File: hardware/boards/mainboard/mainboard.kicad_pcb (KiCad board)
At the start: 2 copper layers, 64.9 x 65 mm, 4 parts, among them J1 Conn_01x03, U1 RP2040

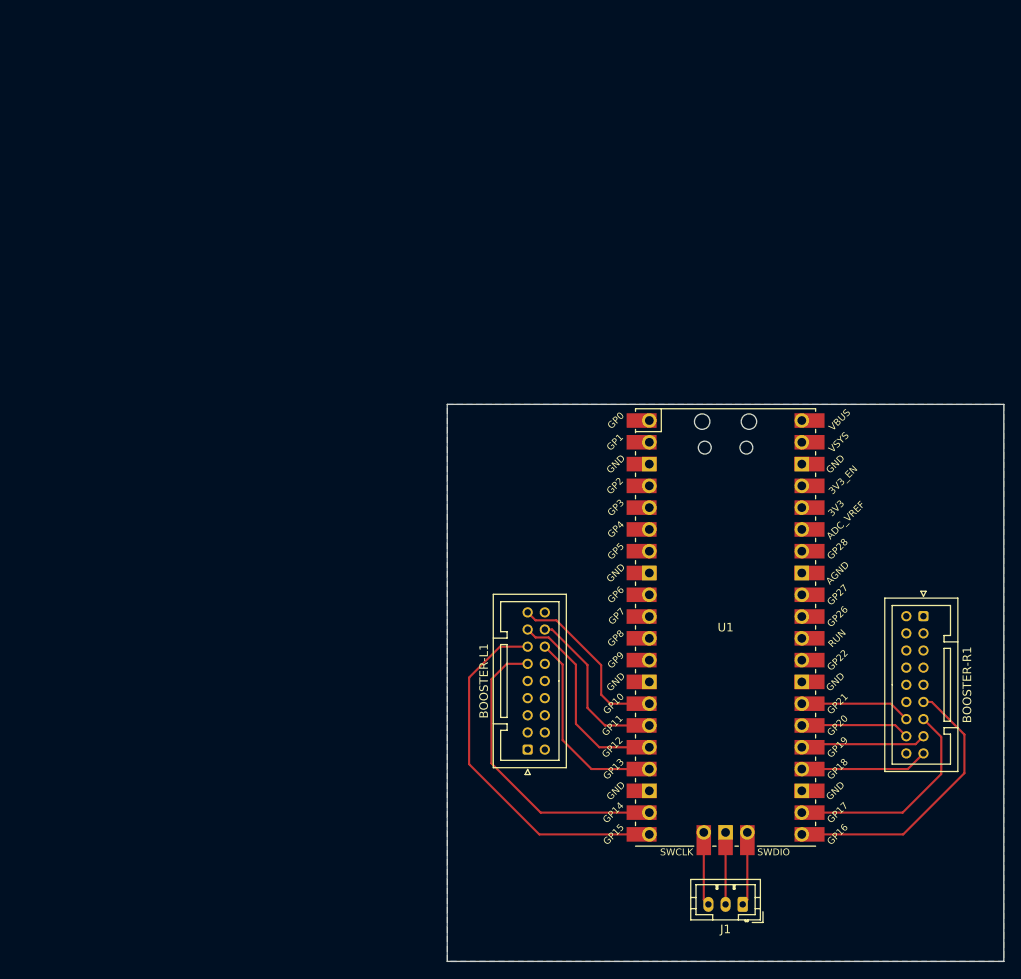
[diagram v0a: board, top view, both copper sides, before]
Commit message: refactor(hardware): refactor mainboard
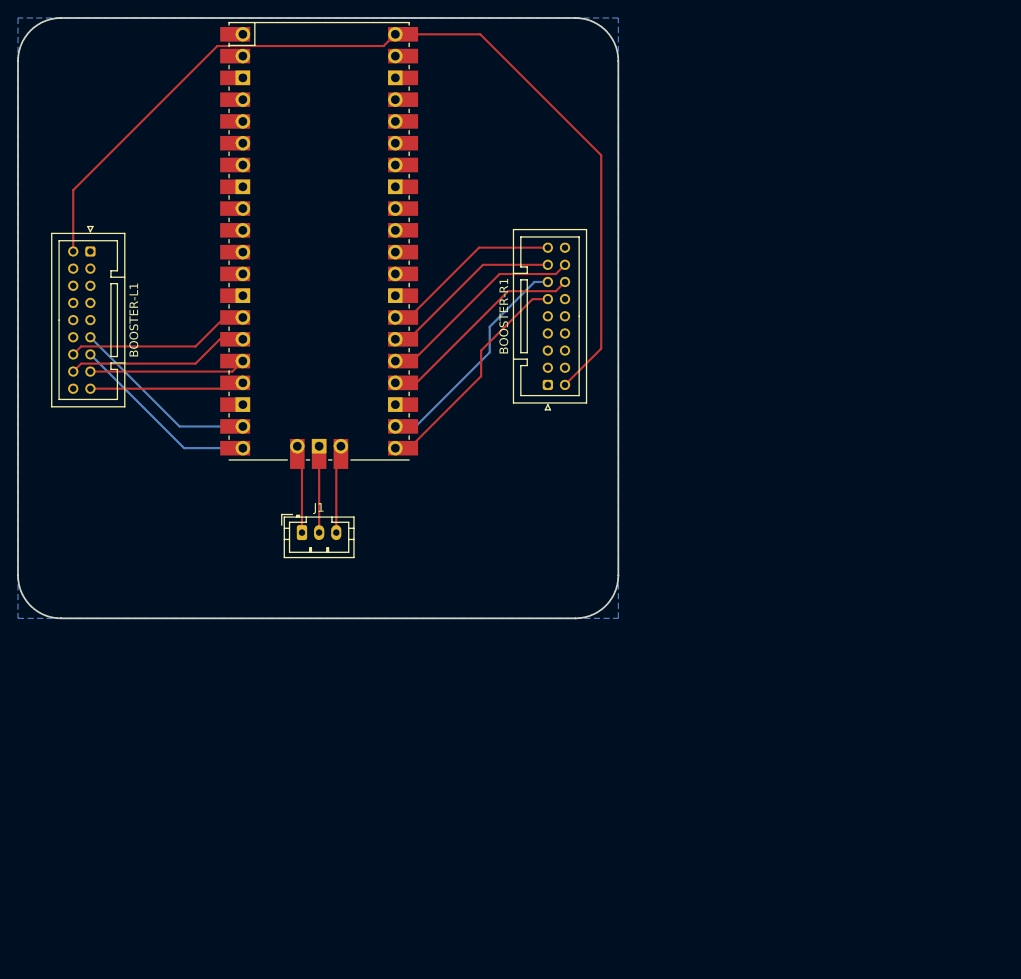
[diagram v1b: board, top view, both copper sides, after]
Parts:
- removed U1: RP2040, MCU_RaspberryPi_and_Boards:RPi_Pico_SMD_TH
- added U2: Pico, MCU_RaspberryPi_and_Boards:RPi_Pico_SMD_TH_Clean, F.Cu at (75.1, 66.0)
- moved BOOSTER-L1 77.3 mm to (48.4, 67.2), turned to -90 degrees
- moved J1 67.2 mm to (73.1, 100.0), turned to 0 degrees
- moved BOOSTER-R1 51.4 mm to (101.8, 82.8), turned to 90 degrees
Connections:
- net BOOSTER_L_SCL+ renamed /BOOSTER_L_SCL+
- net BOOSTER_L_SCL- renamed /BOOSTER_L_SCL-
- net BOOSTER_L_SDA+ renamed /BOOSTER_L_SDA+
- net BOOSTER_L_SDA- renamed /BOOSTER_L_SDA-
- BOOSTER-L1 pad 11: BOOSTER_L_BTN -> /BOOSTER_L_BTN
- BOOSTER-L1 pad 13: BOOSTER_L_BTN_LED -> /BOOSTER_L_BTN_LED
- BOOSTER-L1 pad 14: BOOSTER_L_DIR_4 -> /BOOSTER_L_DIR_4
- BOOSTER-L1 pad 15: BOOSTER_L_DIR_2 -> /BOOSTER_L_DIR_2
- BOOSTER-L1 pad 16: BOOSTER_L_DIR_3 -> /BOOSTER_L_DIR_3
- BOOSTER-L1 pad 17: BOOSTER_L_DIR_1 -> /BOOSTER_L_DIR_1
- BOOSTER-R1 pad 11: BOOSTER_R_BTN -> /BOOSTER_R_BTN
- BOOSTER-R1 pad 13: BOOSTER_R_BTN_LED -> /BOOSTER_R_BTN_LED
- BOOSTER-R1 pad 14: BOOSTER_R_DIR_4 -> /BOOSTER_R_DIR_4
- BOOSTER-R1 pad 15: BOOSTER_R_DIR_2 -> /BOOSTER_R_DIR_2
- BOOSTER-R1 pad 16: BOOSTER_R_DIR_3 -> /BOOSTER_R_DIR_3
- BOOSTER-R1 pad 17: BOOSTER_R_DIR_1 -> /BOOSTER_R_DIR_1
- J1 pad 1: DBG_SWCLK -> /DBG_SWCLK
- J1 pad 2: DBG_GND -> /DBG_GND
- J1 pad 3: DBG_SWDIO -> /DBG_SWDIO
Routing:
- net +5V: track 0.00 -> 110.6 mm
- net BOOSTER_L_BTN_LED: track 42.8 -> 0.00 mm
- net BOOSTER_L_BTN: track 35.6 -> 0.00 mm
- net BOOSTER_R_BTN: track 32.8 -> 0.00 mm
- net /BOOSTER_R_BTN: track 0.00 -> 26.7 mm
- net /BOOSTER_R_BTN_LED: track 0.00 -> 26.5 mm
- net BOOSTER_R_BTN_LED: track 25.4 -> 0.00 mm
- net /BOOSTER_R_DIR_4: track 0.00 -> 24.7 mm
- net /BOOSTER_R_DIR_3: track 0.00 -> 24.4 mm
- net BOOSTER_L_DIR_2: track 23.9 -> 0.00 mm
- net BOOSTER_L_DIR_4: track 23.3 -> 0.00 mm
- net /BOOSTER_L_BTN_LED: track 0.00 -> 22.3 mm
- net /BOOSTER_L_BTN: track 0.00 -> 22.1 mm
- net /BOOSTER_L_DIR_4: track 0.00 -> 21.6 mm
- net /BOOSTER_R_DIR_2: track 0.00 -> 21.4 mm
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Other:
- board size 64.9 x 65 mm -> 70 x 70 mm
